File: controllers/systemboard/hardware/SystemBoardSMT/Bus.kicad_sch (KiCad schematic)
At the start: 1 part, among them U3 VME64-P1-3R

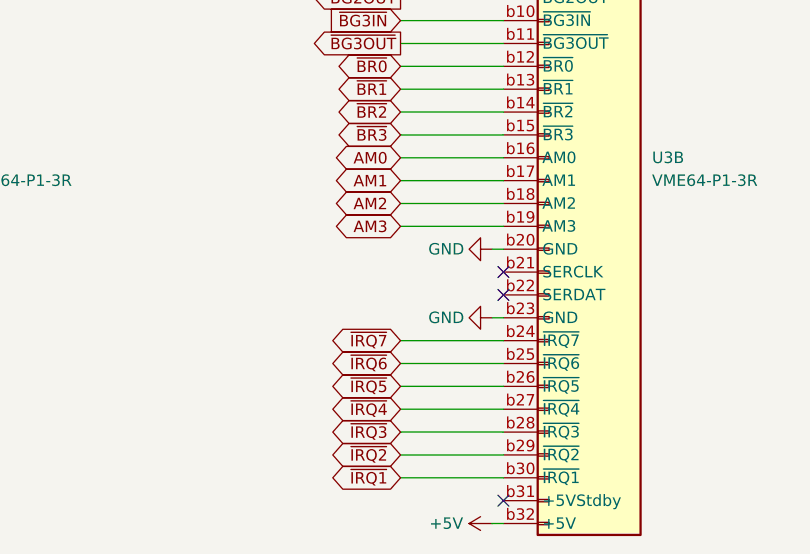
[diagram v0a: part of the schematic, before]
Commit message: Reorganized a bit
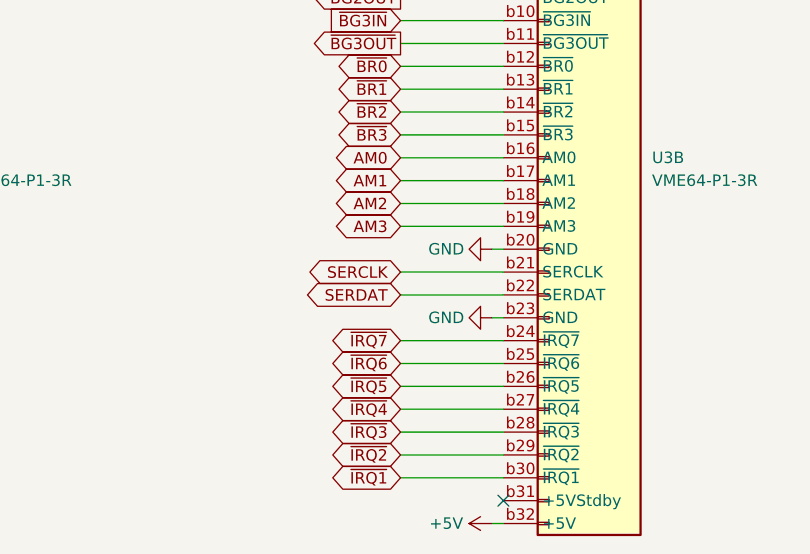
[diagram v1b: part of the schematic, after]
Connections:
- net SERCLK: now reaches U3.b21 (SERCLK)
- net SERDAT: now reaches U3.b22 (SERDAT)
- no-connect marks 13 -> 11
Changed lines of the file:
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@@
-	)
-	(no_connect
-		(at 146.05 80.01)
 	)
 	(no_connect
@@
 	)
 	(no_connect
-		(at 146.05 77.47)
-	)
-	(no_connect
 		(at 233.68 29.21)
 	)
@@
 		)
 	)
+	(wire
+		(pts
+			(xy 134.62 80.01) (xy 146.05 80.01)
+		)
+		(stroke
+			(width 0)
+			(type default)
+		)
+	)
 	(bus
 		(pts
@@
 		(pts
 			(xy 134.62 41.91) (xy 146.05 41.91)
+		)
+		(stroke
+			(width 0)
+			(type default)
+		)
+	)
+	(wire
+		(pts
+			(xy 134.62 77.47) (xy 146.05 77.47)
 		)
 		(stroke
@@
 		)
 	)
+	(global_label "SERDAT"
+		(shape bidirectional)
+		(at 134.62 80.01 180)
+		(fields_autoplaced yes)
+		(effects
+			(font
+				(size 1.27 1.27)
+			)
+			(justify right)
+		)
+		(property "Intersheetrefs" "${INTERSHEET_REFS}"
+			(at 123.5688 80.01 0)
+			(effects
+				(font
+					(size 1.27 1.27)
+				)
+				(justify right)
+				(hide yes)
+			)
+		)
+	)
 	(global_label "AM5"
 		(shape bidirectional)
@@
 			(effects
 				(font
+					(size 1.27 1.27)
+				)
+				(justify right)
+				(hide yes)
+			)
+		)
+	)
+	(global_label "SERCLK"
+		(shape bidirectional)
+		(at 134.62 77.47 180)
+		(fields_autoplaced yes)
+		(effects
+			(font
+				(size 1.27 1.27)
+			)
+			(justify right)
+		)
+		(property "Intersheetrefs" "${INTERSHEET_REFS}"
+			(at 123.3269 77.47 0)
+			(effects
+				(font
